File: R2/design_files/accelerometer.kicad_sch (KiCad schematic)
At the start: 2 parts, among them U12 MC3479

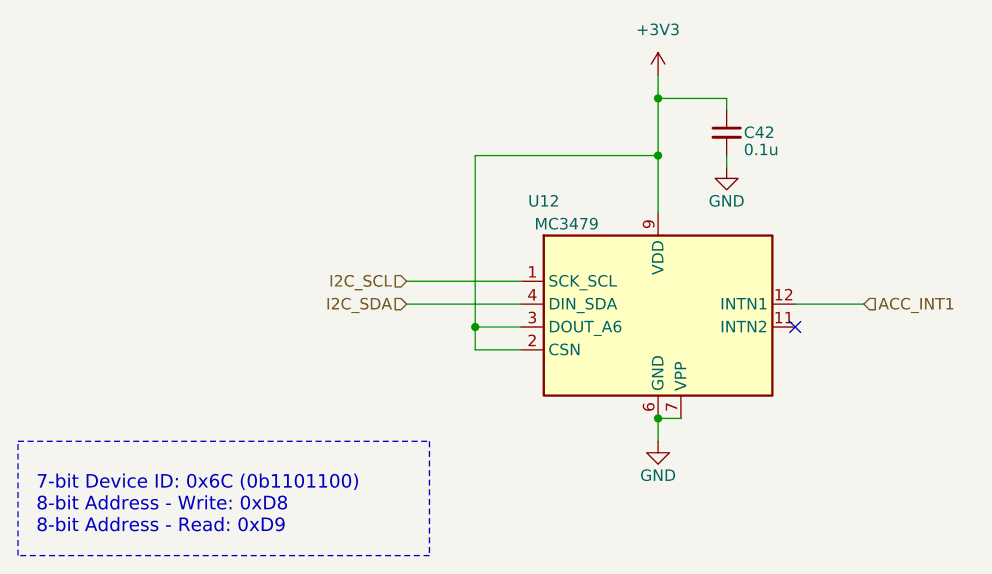
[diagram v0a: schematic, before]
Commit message: Refactor code structure for improved readability and maintainability
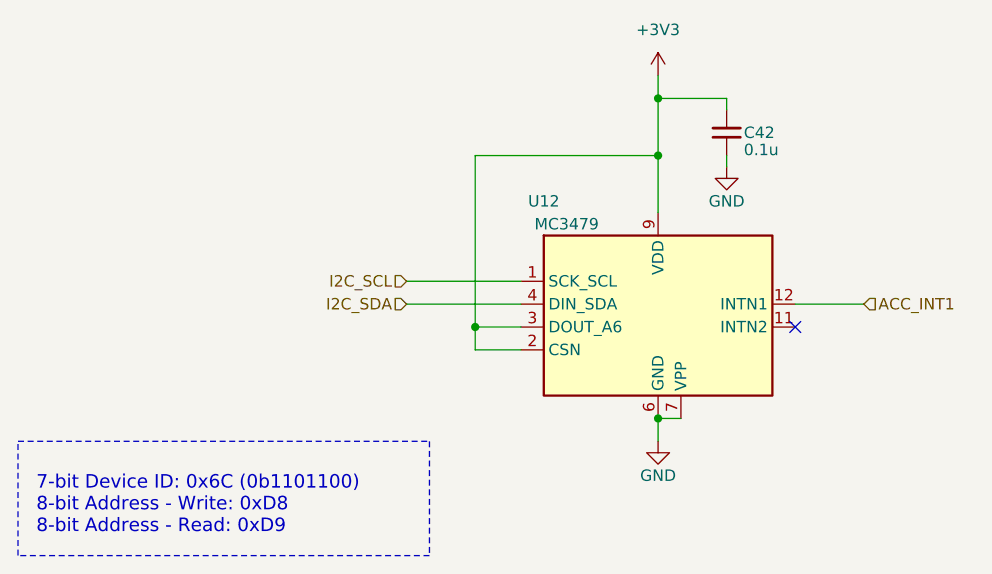
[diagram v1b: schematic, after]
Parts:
- U12: symbol My Libraries:MC3479 -> My_Libraries:MC3479
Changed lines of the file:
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@@
 (kicad_sch
-	(version 20250114)
+	(version 20260306)
 	(generator "eeschema")
-	(generator_version "9.0")
+	(generator_version "10.0")
 	(paper "A4")
 	(title_block
@@
 		(at 157.48 55.88 0)
 		(unit 1)
+		(body_style 1)
 		(exclude_from_sim no)
 		(in_bom yes)
 		(on_board yes)
+		(in_pos_files yes)
 		(dnp no)
 		(fields_autoplaced yes)
 		(property "Reference" "#PWR083"
 			(at 157.48 59.69 0)
-			(effects
-				(font
-					(size 1.27 1.27)
-				)
-				(hide yes)
+			(hide yes)
+			(show_name no)
+			(do_not_autoplace no)
+			(effects
+				(font
+					(size 1.27 1.27)
+				)
 			)
 		)
 		(property "Value" "+3V3"
 			(at 157.48 50.8 0)
+			(show_name no)
+			(do_not_autoplace no)
 			(effects
 				(font
@@
 		(property "Footprint" ""
 			(at 157.48 55.88 0)
-			(effects
-				(font
-					(size 1.27 1.27)
-				)
-				(hide yes)
+			(hide yes)
+			(show_name no)
+			(do_not_autoplace no)
+			(effects
+				(font
+					(size 1.27 1.27)
+				)
 			)
 		)
 		(property "Datasheet" ""
 			(at 157.48 55.88 0)
-			(effects
-				(font
-					(size 1.27 1.27)
-				)
-				(hide yes)
+			(hide yes)
+			(show_name no)
+			(do_not_autoplace no)
+			(effects
+				(font
+					(size 1.27 1.27)
+				)
 			)
 		)
 		(property "Description" "Power symbol creates a global label with name \"+3V3\""
 			(at 157.48 55.88 0)
-			(effects
-				(font
-					(size 1.27 1.27)
-				)
-				(hide yes)
+			(hide yes)
+			(show_name no)
+			(do_not_autoplace no)
+			(effects
+				(font
+					(size 1.27 1.27)
+				)
 			)
 		)
@@
 		(at 165.1 66.04 0)
 		(unit 1)
+		(body_style 1)
 		(exclude_from_sim no)
 		(in_bom yes)
 		(on_board yes)
+		(in_pos_files yes)
 		(dnp no)
 		(property "Reference" "#PWR085"
 			(at 165.1 72.39 0)
-			(effects
-				(font
-					(size 1.27 1.27)
-				)
-				(hide yes)
+			(hide yes)
+			(show_name no)
+			(do_not_autoplace no)
+			(effects
+				(font
+					(size 1.27 1.27)
+				)
 			)
 		)
 		(property "Value" "GND"
 			(at 165.1 69.85 0)
+			(show_name no)
+			(do_not_autoplace no)
 			(effects
 				(font
@@
 		(property "Footprint" ""
 			(at 165.1 66.04 0)
-			(effects
-				(font
-					(size 1.27 1.27)
-				)
-				(hide yes)
+			(hide yes)
+			(show_name no)
+			(do_not_autoplace no)
+			(effects
+				(font
+					(size 1.27 1.27)
+				)
 			)
 		)
 		(property "Datasheet" ""
 			(at 165.1 66.04 0)
-			(effects
-				(font
-					(size 1.27 1.27)
-				)
-				(hide yes)
+			(hide yes)
+			(show_name no)
+			(do_not_autoplace no)
+			(effects
+				(font
+					(size 1.27 1.27)
+				)
 			)
 		)
 		(property "Description" "Power symbol creates a global label with name \"GND\" , ground"
 			(at 165.1 66.04 0)
-			(effects
-				(font
-					(size 1.27 1.27)
-				)
-				(hide yes)
+			(hide yes)
+			(show_name no)
+			(do_not_autoplace no)
+			(effects
+				(font
+					(size 1.27 1.27)
+				)
 			)
 		)
@@
 				)
 			)
-			(project "BK4000TG_V3"
+			(project "tracker"
 				(path "/4f1d18f5-7d2b-4d0b-8633-b1619d53124c/68d45962-0216-4a92-bb54-eaef1d80ce8b"
 					(reference "#PWR085")
@@
 	)
 	(symbol
-		(lib_id "My Libraries:MC3479")
+		(lib_id "My_Libraries:MC3479")
 		(at 157.48 81.28 0)
 		(unit 1)
+		(body_style 1)
 		(exclude_from_sim no)
 		(in_bom yes)
 		(on_board yes)
+		(in_pos_files yes)
 		(dnp no)
 		(property "Reference" "U12"
 			(at 144.78 69.85 0)
+			(show_name no)
+			(do_not_autoplace no)
 			(effects
 				(font
@@
 		(property "Value" "MC3479"
 			(at 147.32 72.39 0)
+			(show_name no)
+			(do_not_autoplace no)
 			(effects
 				(font
@@
 		(property "Footprint" "Package_LGA:LGA-12_2x2mm_P0.5mm"
 			(at 147.32 71.12 0)
-			(effects
-				(font
-					(size 1.27 1.27)
-				)
-				(hide yes)
+			(hide yes)
+			(show_name no)
+			(do_not_autoplace no)
+			(effects
+				(font
+					(size 1.27 1.27)
+				)
 			)
 		)
 		(property "Datasheet" ""
 			(at 147.32 71.12 0)
-			(effects
-				(font
-					(size 1.27 1.27)
-				)
-				(hide yes)
+			(hide yes)
+			(show_name no)
+			(do_not_autoplace no)
+			(effects
+				(font
+					(size 1.27 1.27)
+				)
 			)
 		)
 		(property "Description" "3-Axis Accelerometer ±2, ±4, ±8, ±12, ±16g range 16-bit 4 μA, SPI, I2C"
 			(at 157.48 81.28 0)
-			(effects
-				(font
-					(size 1.27 1.27)
-				)
-				(hide yes)
+			(hide yes)
+			(show_name no)
+			(do_not_autoplace no)
+			(effects
+				(font
+					(size 1.27 1.27)
+				)
 			)
 		)
@@
 				)
 			)
-			(project "BK4000TG_V3"
+			(project "tracker"
 				(path "/4f1d18f5-7d2b-4d0b-8633-b1619d53124c/68d45962-0216-4a92-bb54-eaef1d80ce8b"
 					(reference "U12")
@@
 		(at 165.1 62.23 0)
 		(unit 1)
+		(body_style 1)
 		(exclude_from_sim no)
 		(in_bom yes)
 		(on_board yes)
+		(in_pos_files yes)
 		(dnp no)
 		(property "Reference" "C42"
 			(at 167.005 62.2299 0)
+			(show_name no)
+			(do_not_autoplace no)
 			(effects
 				(font
@@
 		(property "Value" "0.1u"
 			(at 167.005 64.1349 0)
+			(show_name no)
+			(do_not_autoplace no)
 			(effects
 				(font
@@
 		(property "Footprint" "Capacitor_SMD:C_0603_1608Metric"
 			(at 165.1 62.23 0)
-			(effects
-				(font
-					(size 1.27 1.27)
-				)
-				(hide yes)
-			)
-		)
-		(property "Datasheet" "~"
+			(hide yes)
+			(show_name no)
+			(do_not_autoplace no)
+			(effects
+				(font
+					(size 1.27 1.27)
+				)
+			)
+		)
+		(property "Datasheet" ""
 			(at 165.1 62.23 0)
-			(effects
-				(font
-					(size 1.27 1.27)
-				)
-				(hide yes)
+			(hide yes)
+			(show_name no)
+			(do_not_autoplace no)
+			(effects
+				(font
+					(size 1.27 1.27)
+				)
 			)
 		)
 		(property "Description" "Unpolarized capacitor, small symbol"
 			(at 165.1 62.23 0)
-			(effects
-				(font
-					(size 1.27 1.27)
-				)
-				(hide yes)
+			(hide yes)
+			(show_name no)
+			(do_not_autoplace no)
+			(effects
+				(font
+					(size 1.27 1.27)
+				)
 			)
 		)
@@
 				)
 			)
-			(project "BK4000TG_V3"
+			(project "tracker"
 				(path "/4f1d18f5-7d2b-4d0b-8633-b1619d53124c/68d45962-0216-4a92-bb54-eaef1d80ce8b"
 					(reference "C42")
@@
 		(at 157.48 96.52 0)
 		(unit 1)
+		(body_style 1)
 		(exclude_from_sim no)
 		(in_bom yes)
 		(on_board yes)
+		(in_pos_files yes)
 		(dnp no)
 		(property "Reference" "#PWR084"
 			(at 157.48 102.87 0)
-			(effects
-				(font
-					(size 1.27 1.27)
-				)
-				(hide yes)
+			(hide yes)
+			(show_name no)
+			(do_not_autoplace no)
+			(effects
+				(font
+					(size 1.27 1.27)
+				)
 			)
 		)
 		(property "Value" "GND"
 			(at 157.48 100.33 0)
+			(show_name no)
+			(do_not_autoplace no)
 			(effects
 				(font
@@
 		(property "Footprint" ""
 			(at 157.48 96.52 0)
-			(effects
-				(font
-					(size 1.27 1.27)
-				)
-				(hide yes)
+			(hide yes)
+			(show_name no)
+			(do_not_autoplace no)
+			(effects
+				(font
+					(size 1.27 1.27)
+				)
 			)
 		)
 		(property "Datasheet" ""
 			(at 157.48 96.52 0)
-			(effects
-				(font
-					(size 1.27 1.27)
-				)
-				(hide yes)
+			(hide yes)
+			(show_name no)
+			(do_not_autoplace no)
+			(effects
+				(font
+					(size 1.27 1.27)
+				)
 			)
 		)
 		(property "Description" "Power symbol creates a global label with name \"GND\" , ground"
 			(at 157.48 96.52 0)
-			(effects
-				(font
-					(size 1.27 1.27)
-				)
-				(hide yes)
+			(hide yes)
+			(show_name no)
+			(do_not_autoplace no)
+			(effects
+				(font
+					(size 1.27 1.27)
+				)
 			)
 		)
@@
 				)
 			)
-			(project "BK4000TG_V3"
+			(project "tracker"
 				(path "/4f1d18f5-7d2b-4d0b-8633-b1619d53124c/68d45962-0216-4a92-bb54-eaef1d80ce8b"
 					(reference "#PWR084")
